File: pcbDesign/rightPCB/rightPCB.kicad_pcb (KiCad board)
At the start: 4 copper layers, 58.5 x 90 mm, 13 parts, among them J1 Conn_01x07_Pin, SW5 RotaryEncoder, SW6 TL, SW7 TR, SW8 PS

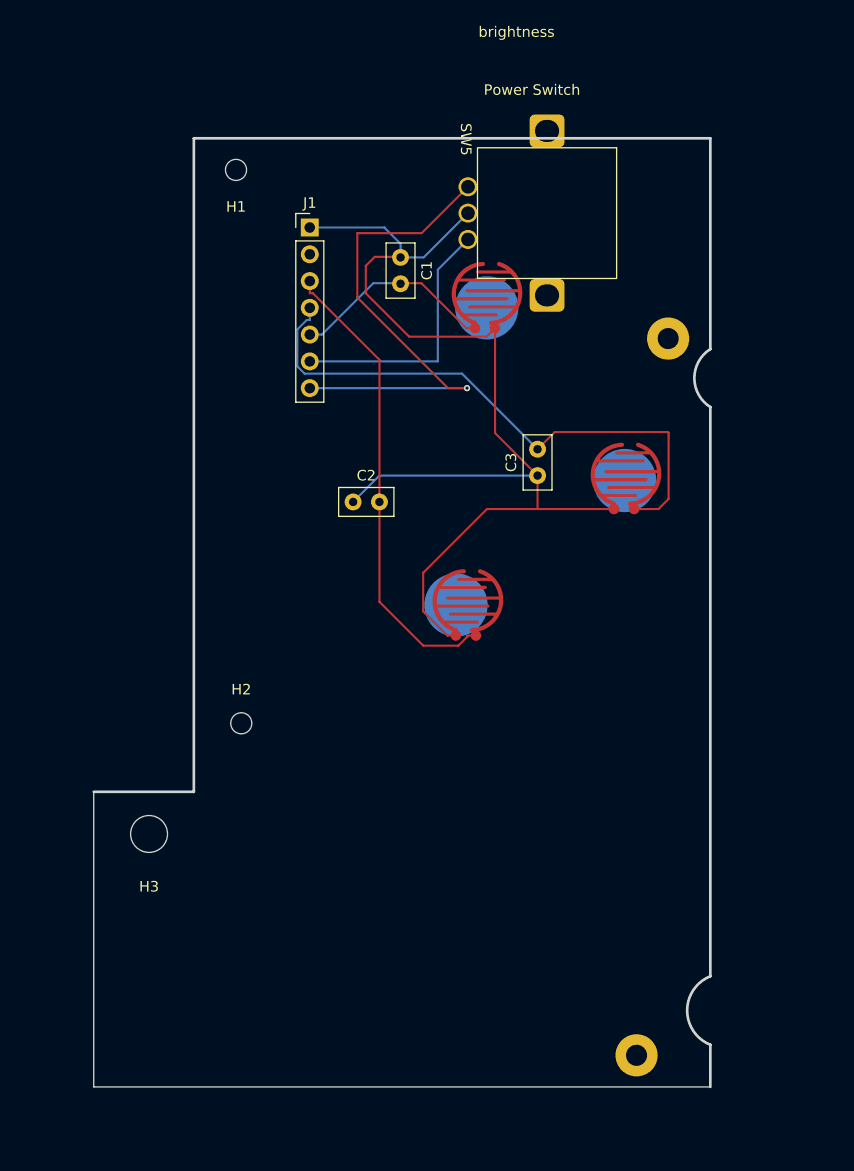
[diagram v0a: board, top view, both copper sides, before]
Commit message: right pcb edits
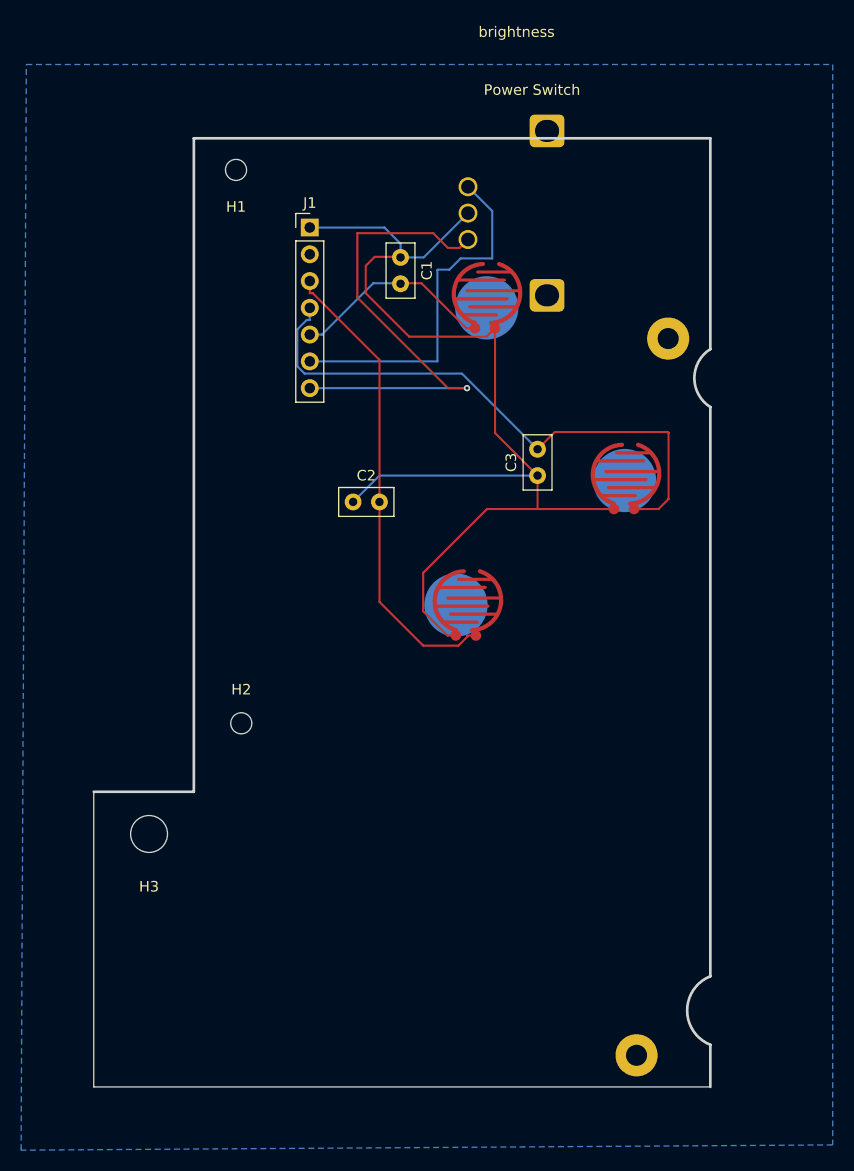
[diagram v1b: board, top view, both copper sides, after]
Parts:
- SW5: moved to B.Cu
- moved SW5 12.4 mm to (229.5, 73.3), turned to 90 degrees
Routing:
- net /Brightness_B: track 24.9 -> 34.2 mm
- net /Brightness_A: track 47.3 -> 46.4 mm
- added copper zone on B.Cu, net GND
- removed copper zone on In1.Cu, net GND
- removed copper zone on In2.Cu, net GND
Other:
- copper layers 4 -> 2
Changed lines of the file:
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@@
 	(layers
 		(0 "F.Cu" signal "TopLayer")
-		(4 "In1.Cu" signal)
-		(6 "In2.Cu" signal)
 		(2 "B.Cu" signal "BottomLayer")
 		(9 "F.Adhes" user "F.Adhesive")
@@
 			)
 			(layer "dielectric 1"
-				(type "prepreg")
-				(thickness 0.1)
-				(material "FR4")
-				(epsilon_r 4.5)
-				(loss_tangent 0.02)
-			)
-			(layer "In1.Cu"
-				(type "copper")
-				(thickness 0.035)
-			)
-			(layer "dielectric 2"
 				(type "core")
-				(thickness 1.24)
-				(material "FR4")
-				(epsilon_r 4.5)
-				(loss_tangent 0.02)
-			)
-			(layer "In2.Cu"
-				(type "copper")
-				(thickness 0.035)
-			)
-			(layer "dielectric 3"
-				(type "prepreg")
-				(thickness 0.1)
+				(thickness 1.51)
 				(material "FR4")
 				(epsilon_r 4.5)
@@
 		(embedded_fonts no)
 	)
-	(footprint "GGLib:PES12"
-		(layer "F.Cu")
-		(at 229.5 60.9 -90)
-		(property "Reference" "SW5"
-			(at -0.8 14.3 270)
-			(unlocked yes)
-			(layer "F.SilkS")
-			(effects
-				(font
-					(size 1 1)
-					(thickness 0.1)
-				)
-			)
-		)
-		(property "Value" "RotaryEncoder"
-			(at 1.7 17.3 270)
-			(unlocked yes)
-			(layer "F.Fab")
-			(effects
-				(font
-					(size 1 1)
-					(thickness 0.15)
-				)
-			)
-		)
-		(property "Datasheet" ""
-			(at 0 0 270)
-			(unlocked yes)
-			(layer "F.Fab")
-			(hide yes)
-			(effects
-				(font
-					(size 1 1)
-					(thickness 0.15)
-				)
-			)
-		)
-		(property "Description" "Rotary encoder, dual channel, incremental quadrate outputs"
-			(at 0 0 270)
-			(unlocked yes)
-			(layer "F.Fab")
-			(hide yes)
-			(effects
-				(font
-					(size 1 1)
-					(thickness 0.15)
-				)
-			)
-		)
-		(property ki_fp_filters "RotaryEncoder*")
-		(sheetname "/")
-		(sheetfile "rightPCB.kicad_sch")
-		(attr smd)
-		(fp_rect
-			(start 0 0)
-			(end 12.4 13.2)
-			(stroke
-				(width 0.1)
-				(type solid)
-			)
-			(fill no)
-			(layer "F.SilkS")
-		)
-		(pad "" thru_hole roundrect
-			(at -1.6 6.6 270)
-			(size 3.1 3.3)
-			(drill oval 2.1 2.3)
-			(layers "*.Cu" "*.Mask")
-			(remove_unused_layers no)
-			(roundrect_rratio 0.15)
-			(thermal_bridge_angle 45)
-		)
-		(pad "" thru_hole roundrect
-			(at 14 6.6 270)
-			(size 3.1 3.3)
-			(drill oval 2.1 2.3)
-			(layers "*.Cu" "*.Mask")
-			(remove_unused_layers no)
-			(roundrect_rratio 0.15)
-			(thermal_bridge_angle 45)
-		)
-		(pad "A" thru_hole circle
-			(at 3.7 14.1 270)
-			(size 1.8 1.8)
-			(drill 1.3)
-			(layers "*.Cu" "*.Mask")
-			(remove_unused_layers no)
-			(net 6 "/Brightness_A")
-			(pinfunction "A")
-			(pintype "passive")
-		)
-		(pad "B" thru_hole circle
-			(at 8.7 14.1 270)
-			(size 1.8 1.8)
-			(drill 1.3)
-			(layers "*.Cu" "*.Mask")
-			(remove_unused_layers no)
-			(net 7 "/Brightness_B")
-			(pinfunction "B")
-			(pintype "passive")
-		)
-		(pad "C" thru_hole circle
-			(at 6.2 14.1 270)
-			(size 1.8 1.8)
-			(drill 1.3)
-			(layers "*.Cu" "*.Mask")
-			(remove_unused_layers no)
-			(net 1 "GND")
-			(pinfunction "C")
-			(pintype "passive")
-		)
-		(embedded_fonts no)
-	)
 	(footprint "MountingHole:MountingHole_2mm"
 		(layer "F.Cu")
@@
 		)
 	)
+	(footprint "GGLib:PES12"
+		(layer "B.Cu")
+		(at 229.5 73.3 90)
+		(property "Reference" "SW5"
+			(at -0.8 -14.3 270)
+			(unlocked yes)
+			(layer "B.SilkS")
+			(effects
+				(font
+					(size 1 1)
+					(thickness 0.1)
+				)
+				(justify mirror)
+			)
+		)
+		(property "Value" "RotaryEncoder"
+			(at 1.7 -17.3 270)
+			(unlocked yes)
+			(layer "B.Fab")
+			(effects
+				(font
+					(size 1 1)
+					(thickness 0.15)
+				)
+				(justify mirror)
+			)
+		)
+		(property "Datasheet" ""
+			(at 0 0 270)
+			(unlocked yes)
+			(layer "B.Fab")
+			(hide yes)
+			(effects
+				(font
+					(size 1 1)
+					(thickness 0.15)
+				)
+				(justify mirror)
+			)
+		)
+		(property "Description" "Rotary encoder, dual channel, incremental quadrate outputs"
+			(at 0 0 270)
+			(unlocked yes)
+			(layer "B.Fab")
+			(hide yes)
+			(effects
+				(font
+					(size 1 1)
+					(thickness 0.15)
+				)
+				(justify mirror)
+			)
+		)
+		(property ki_fp_filters "RotaryEncoder*")
+		(sheetname "/")
+		(sheetfile "rightPCB.kicad_sch")
+		(attr smd)
+		(fp_rect
+			(start 0 0)
+			(end 12.4 -13.2)
+			(stroke
+				(width 0.1)
+				(type solid)
+			)
+			(fill no)
+			(layer "B.SilkS")
+		)
+		(pad "" thru_hole roundrect
+			(at -1.6 -6.6 90)
+			(size 3.1 3.3)
+			(drill oval 2.1 2.3)
+			(layers "*.Cu" "*.Mask")
+			(remove_unused_layers no)
+			(roundrect_rratio 0.15)
+			(thermal_bridge_angle 45)
+		)
+		(pad "" thru_hole roundrect
+			(at 14 -6.6 90)
+			(size 3.1 3.3)
+			(drill oval 2.1 2.3)
+			(layers "*.Cu" "*.Mask")
+			(remove_unused_layers no)
+			(roundrect_rratio 0.15)
+			(thermal_bridge_angle 45)
+		)
+		(pad "A" thru_hole circle
+			(at 3.7 -14.1 90)
+			(size 1.8 1.8)
+			(drill 1.3)
+			(layers "*.Cu" "*.Mask")
+			(remove_unused_layers no)
+			(net 6 "/Brightness_A")
+			(pinfunction "A")
+			(pintype "passive")
+		)
+		(pad "B" thru_hole circle
+			(at 8.7 -14.1 90)
+			(size 1.8 1.8)
+			(drill 1.3)
+			(layers "*.Cu" "*.Mask")
+			(remove_unused_layers no)
+			(net 7 "/Brightness_B")
+			(pinfunction "B")
+			(pintype "passive")
+		)
+		(pad "C" thru_hole circle
+			(at 6.2 -14.1 90)
+			(size 1.8 1.8)
+			(drill 1.3)
+			(layers "*.Cu" "*.Mask")
+			(remove_unused_layers no)
+			(net 1 "GND")
+			(pinfunction "C")
+			(pintype "passive")
+		)
+		(embedded_fonts no)
+	)
 	(footprint "BackupProjects_allisonbarfield_personal_3_20250219:Pad_gge24780"
 		(locked yes)
@@
 	)
 	(segment
+		(start 213.5 70.4)
+		(end 214.6 70.4)
+		(width 0.2)
+		(layer "F.Cu")
+		(net 6)
+	)
+	(segment
+		(start 204.9 69)
+		(end 212.1 69)
+		(width 0.2)
+		(layer "F.Cu")
+		(net 6)
+	)
+	(segment
+		(start 204.9 75.1)
+		(end 204.9 69)
+		(width 0.2)
+		(layer "F.Cu")
+		(net 6)
+	)
+	(segment
+		(start 214.6 70.4)
+		(end 215.4 69.6)
+		(width 0.2)
+		(layer "F.Cu")
+		(net 6)
+	)
+	(segment
 		(start 213.5041 83.7041)
 		(end 204.9 75.1)
@@
 	)
 	(segment
-		(start 211 69)
-		(end 215.4 64.6)
-		(width 0.2)
-		(layer "F.Cu")
-		(net 6)
-	)
-	(segment
-		(start 204.9 75.1)
-		(end 204.9 69)
-		(width 0.2)
-		(layer "F.Cu")
-		(net 6)
-	)
-	(segment
 		(start 215.3076 83.7041)
 		(end 213.5041 83.7041)
@@
 	)
 	(segment
-		(start 204.9 69)
-		(end 211 69)
+		(start 212.1 69)
+		(end 213.5 70.4)
 		(width 0.2)
 		(layer "F.Cu")
@@
 	)
 	(segment
+		(start 217.7 71.4)
+		(end 217.7 66.9)
+		(width 0.2)
+		(layer "B.Cu")
+		(net 7)
+	)
+	(segment
+		(start 212.5 81.1641)
+		(end 212.5 72.5)
+		(width 0.2)
+		(layer "B.Cu")
+		(net 7)
+	)
+	(segment
 		(start 200.3906 81.1641)
-		(end 212.5359 81.1641)
+		(end 212.5 81.1641)
 		(width 0.2)
 		(layer "B.Cu")
@@
 	)
 	(segment
-		(start 212.5359 81.1641)
+		(start 217.7 66.9)
+		(end 215.4 64.6)
+		(width 0.2)
+		(layer "B.Cu")
+		(net 7)
+	)
+	(segment
+		(start 213.6359 72.4641)
+		(end 214.7 71.4)
+		(width 0.2)
+		(layer "B.Cu")
+		(net 7)
+	)
+	(segment
+		(start 214.7 71.4)
+		(end 217.7 71.4)
+		(width 0.2)
+		(layer "B.Cu")
+		(net 7)
+	)
+	(segment
+		(start 212.5 72.5)
 		(end 212.5359 72.4641)
 		(width 0.2)
@@
 	(segment
 		(start 212.5359 72.4641)
-		(end 215.4 69.6)
+		(end 213.6359 72.4641)
 		(width 0.2)
 		(layer "B.Cu")
@@
 		(net 1)
 		(net_name "GND")
-		(layer "In1.Cu")
+		(layer "B.Cu")
 		(hatch edge 0.5)
 		(connect_pads
@@
 		(polygon
 			(pts
-				(xy 174 58) (xy 241.5 58) (xy 241.5 152) (xy 174 152)
-			)
-		)
-	)
-	(zone
-		(net 1)
-		(net_name "GND")
-		(layer "In2.Cu")
-		(hatch edge 0.5)
-		(priority 1)
-		(connect_pads
-			(clearance 0.5)
-		)
-		(min_thickness 0.25)
-		(filled_areas_thickness no)
-		(fill yes
-			(thermal_gap 0.5)
-			(thermal_bridge_width 0.5)
-		)
-		(polygon
-			(pts
-				(xy 174 58) (xy 241.5 58) (xy 241.5 152) (xy 174 152.5)
-			)
-		)
+				(xy 173.5 53) (xy 250 53) (xy 250 155.5) (xy 173 156)
+			)
+		)
